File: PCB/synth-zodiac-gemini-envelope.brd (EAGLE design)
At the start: 76.1 x 72.4 mm, 23 parts, among them Q1 PNP, U1 TL074A

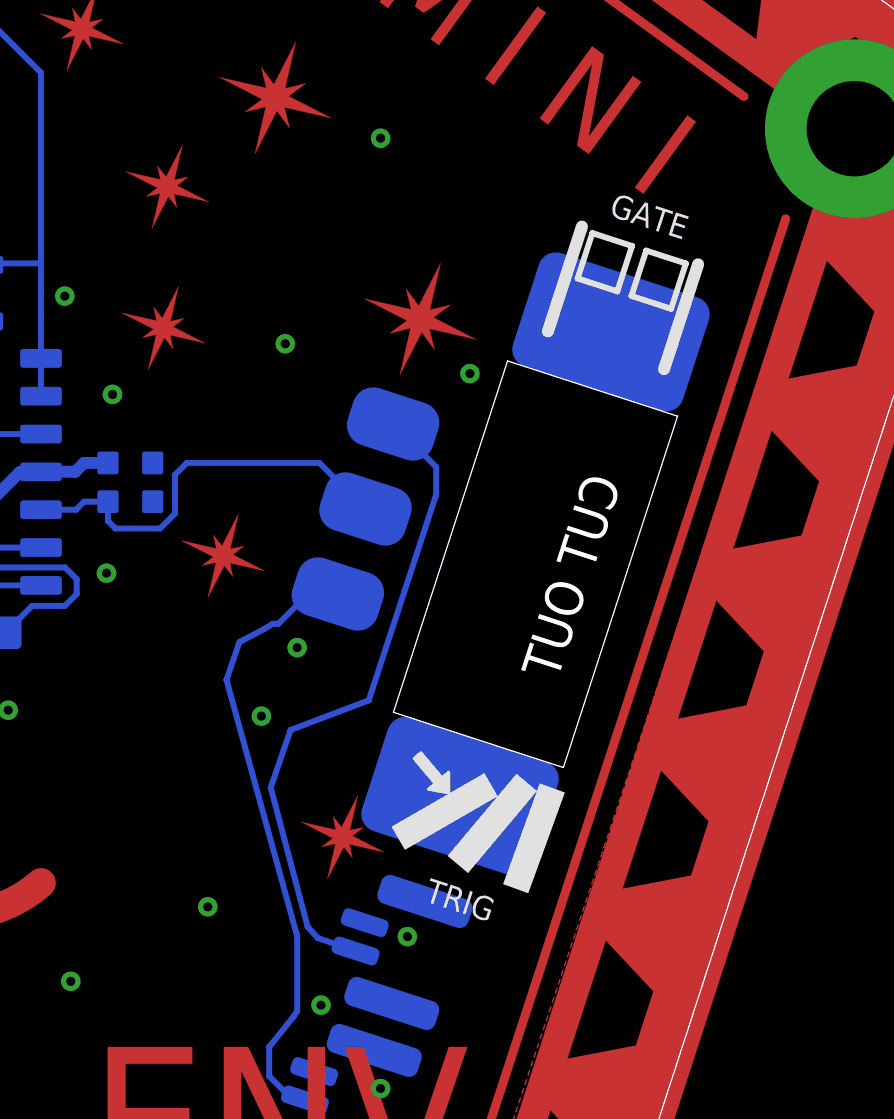
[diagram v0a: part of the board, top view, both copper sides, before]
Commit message: Perhaps final Rev. A?
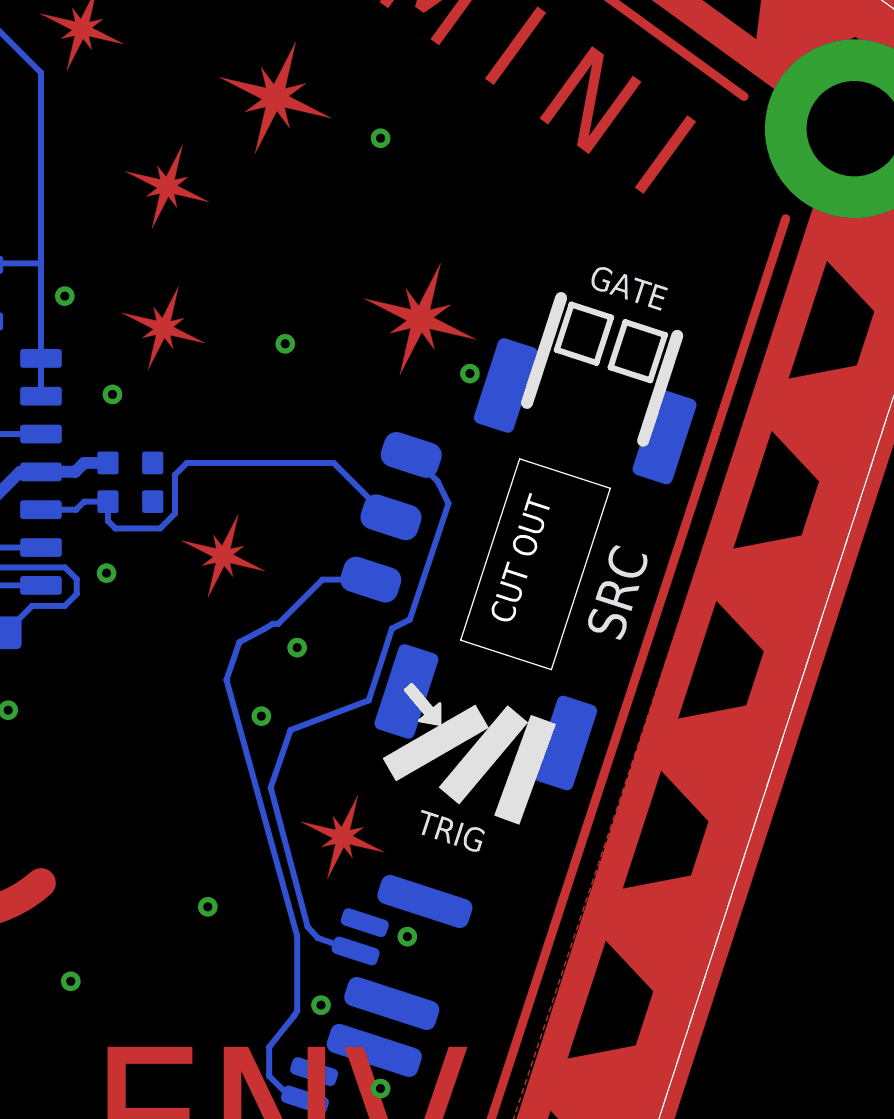
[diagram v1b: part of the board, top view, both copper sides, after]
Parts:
- SRC: device switch-thd:SS-12-F45-PNL-SMT -> switch-thd:SS-12-F45-PNL-SMT-2
- flipped SRC to the top, turned to 252 degrees
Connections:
- net GATE: now also SRC.A; no longer SRC.B
- net GND: now also SRC.MTG3, SRC.MTG4
- net TRIG: now also SRC.B; no longer SRC.A
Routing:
- net TRIG: track 20.7 -> 22.0 mm
- net N$134: track 14.1 -> 15.0 mm
- net GATE: track 21.8 -> 20.9 mm

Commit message: Tune values and some schematic visual tweaks.
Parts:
- C1: value 1.0uF -> 1.0uF/16V
- C2: value 2.2uF -> 2.2uF/16V
- C3, C4: value 0.1uF -> 0.1uF/16V
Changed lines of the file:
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@@
 <attribute name="VALUE" x="41.2" y="32.3" size="0.4064" layer="28" font="vector" rot="MR90" align="center"/>
 </element>
-<element name="C1" library="rlc" library_urn="urn:adsk.eagle:library:4192893" package="0603-CAP" package3d_urn="urn:adsk.eagle:package:4193021/4" value="1.0uF" x="33.9" y="30.9" smashed="yes" rot="MR0">
+<element name="C1" library="rlc" library_urn="urn:adsk.eagle:library:4192893" package="0603-CAP" package3d_urn="urn:adsk.eagle:package:4193021/4" value="1.0uF/16V" x="33.9" y="30.9" smashed="yes" rot="MR0">
 <attribute name="COST01" value="0.12" x="33.9" y="30.9" size="1.778" layer="28" rot="MR0" display="off"/>
 <attribute name="COST10" value="0.09" x="33.9" y="30.9" size="1.778" layer="28" rot="MR0" display="off"/>
@@
 <attribute name="VALUE" x="31.25" y="35.4" size="0.3048" layer="28" font="vector" rot="MR0" align="center"/>
 </element>
-<element name="C2" library="rlc" library_urn="urn:adsk.eagle:library:4192893" package="0603-CAP" package3d_urn="urn:adsk.eagle:package:4193021/4" value="2.2uF" x="32.6" y="38.5" smashed="yes" rot="MR0">
+<element name="C2" library="rlc" library_urn="urn:adsk.eagle:library:4192893" package="0603-CAP" package3d_urn="urn:adsk.eagle:package:4193021/4" value="2.2uF/16V" x="32.6" y="38.5" smashed="yes" rot="MR0">
 <attribute name="COST01" value="0.12" x="32.6" y="38.5" size="1.778" layer="28" rot="MR0" display="off"/>
 <attribute name="COST10" value="0.09" x="32.6" y="38.5" size="1.778" layer="28" rot="MR0" display="off"/>
@@
 <attribute name="VALUE" x="33.9" y="27.3" size="0.2" layer="28" rot="MR180" align="center"/>
 </element>
-<element name="C3" library="rlc" library_urn="urn:adsk.eagle:library:4192893" package="0603-CAP" package3d_urn="urn:adsk.eagle:package:4193021/4" value="0.1uF" x="47" y="32.6" smashed="yes" rot="MR180">
+<element name="C3" library="rlc" library_urn="urn:adsk.eagle:library:4192893" package="0603-CAP" package3d_urn="urn:adsk.eagle:package:4193021/4" value="0.1uF/16V" x="47" y="32.6" smashed="yes" rot="MR180">
 <attribute name="COST01" value="0.12" x="47" y="32.6" size="1.778" layer="28" rot="MR180" display="off"/>
 <attribute name="COST10" value="0.09" x="47" y="32.6" size="1.778" layer="28" rot="MR180" display="off"/>
@@
 <attribute name="VALUE" x="47" y="32.6" size="0.2" layer="28" rot="MR180" align="center"/>
 </element>
-<element name="C4" library="rlc" library_urn="urn:adsk.eagle:library:4192893" package="0603-CAP" package3d_urn="urn:adsk.eagle:package:4193021/4" value="0.1uF" x="33.9" y="29.7" smashed="yes" rot="MR180">
+<element name="C4" library="rlc" library_urn="urn:adsk.eagle:library:4192893" package="0603-CAP" package3d_urn="urn:adsk.eagle:package:4193021/4" value="0.1uF/16V" x="33.9" y="29.7" smashed="yes" rot="MR180">
 <attribute name="COST01" value="0.12" x="33.9" y="29.7" size="1.778" layer="28" rot="MR180" display="off"/>
 <attribute name="COST10" value="0.09" x="33.9" y="29.7" size="1.778" layer="28" rot="MR180" display="off"/>
